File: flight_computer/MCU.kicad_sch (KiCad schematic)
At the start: 43 parts, among them J1 Conn_02x05_Odd_Even, J2 MEM2061-01-188-00-A_REVA, Q1 Q_NPN_BEC, SW1 SW_Push, SW2 SW_Push, U2 STM8S007C8T6TR, Y1 12MHz

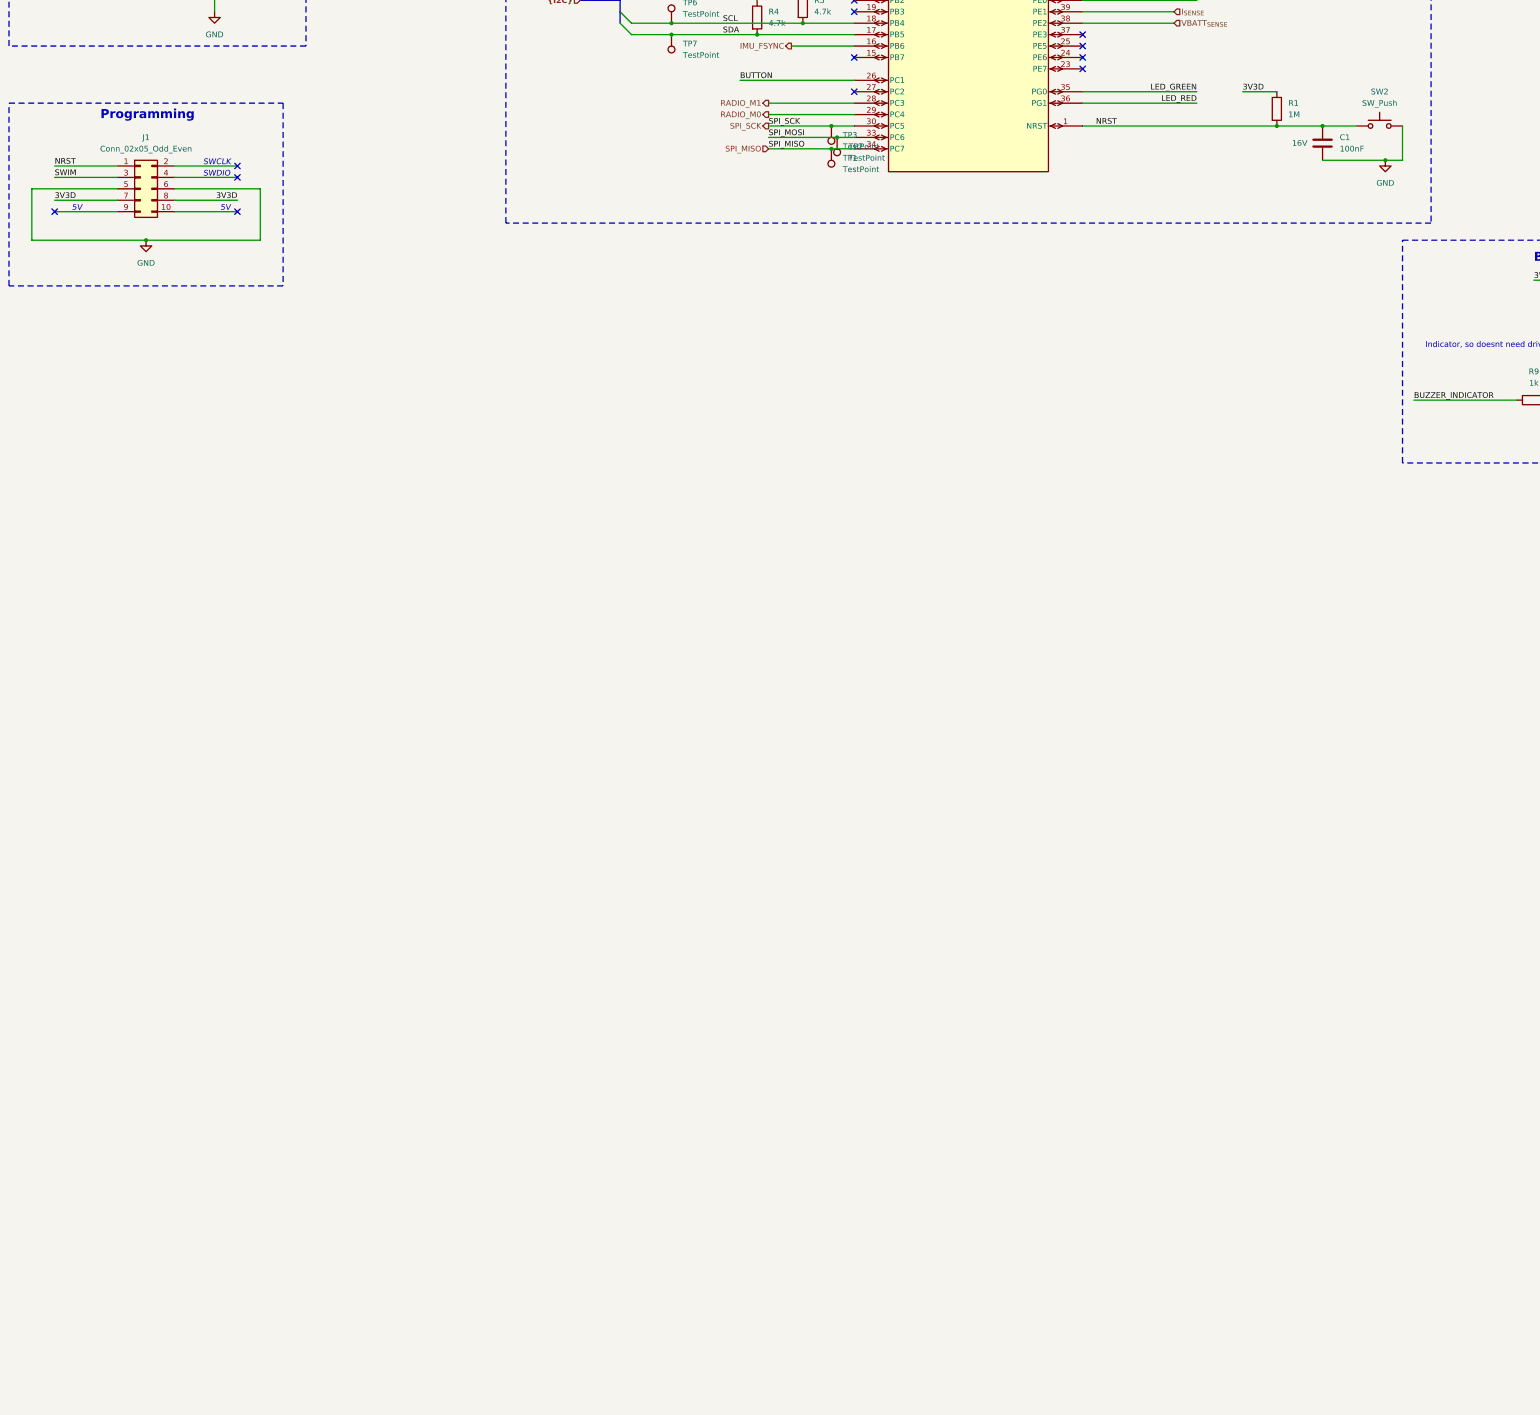
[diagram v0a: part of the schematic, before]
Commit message: start of esp32
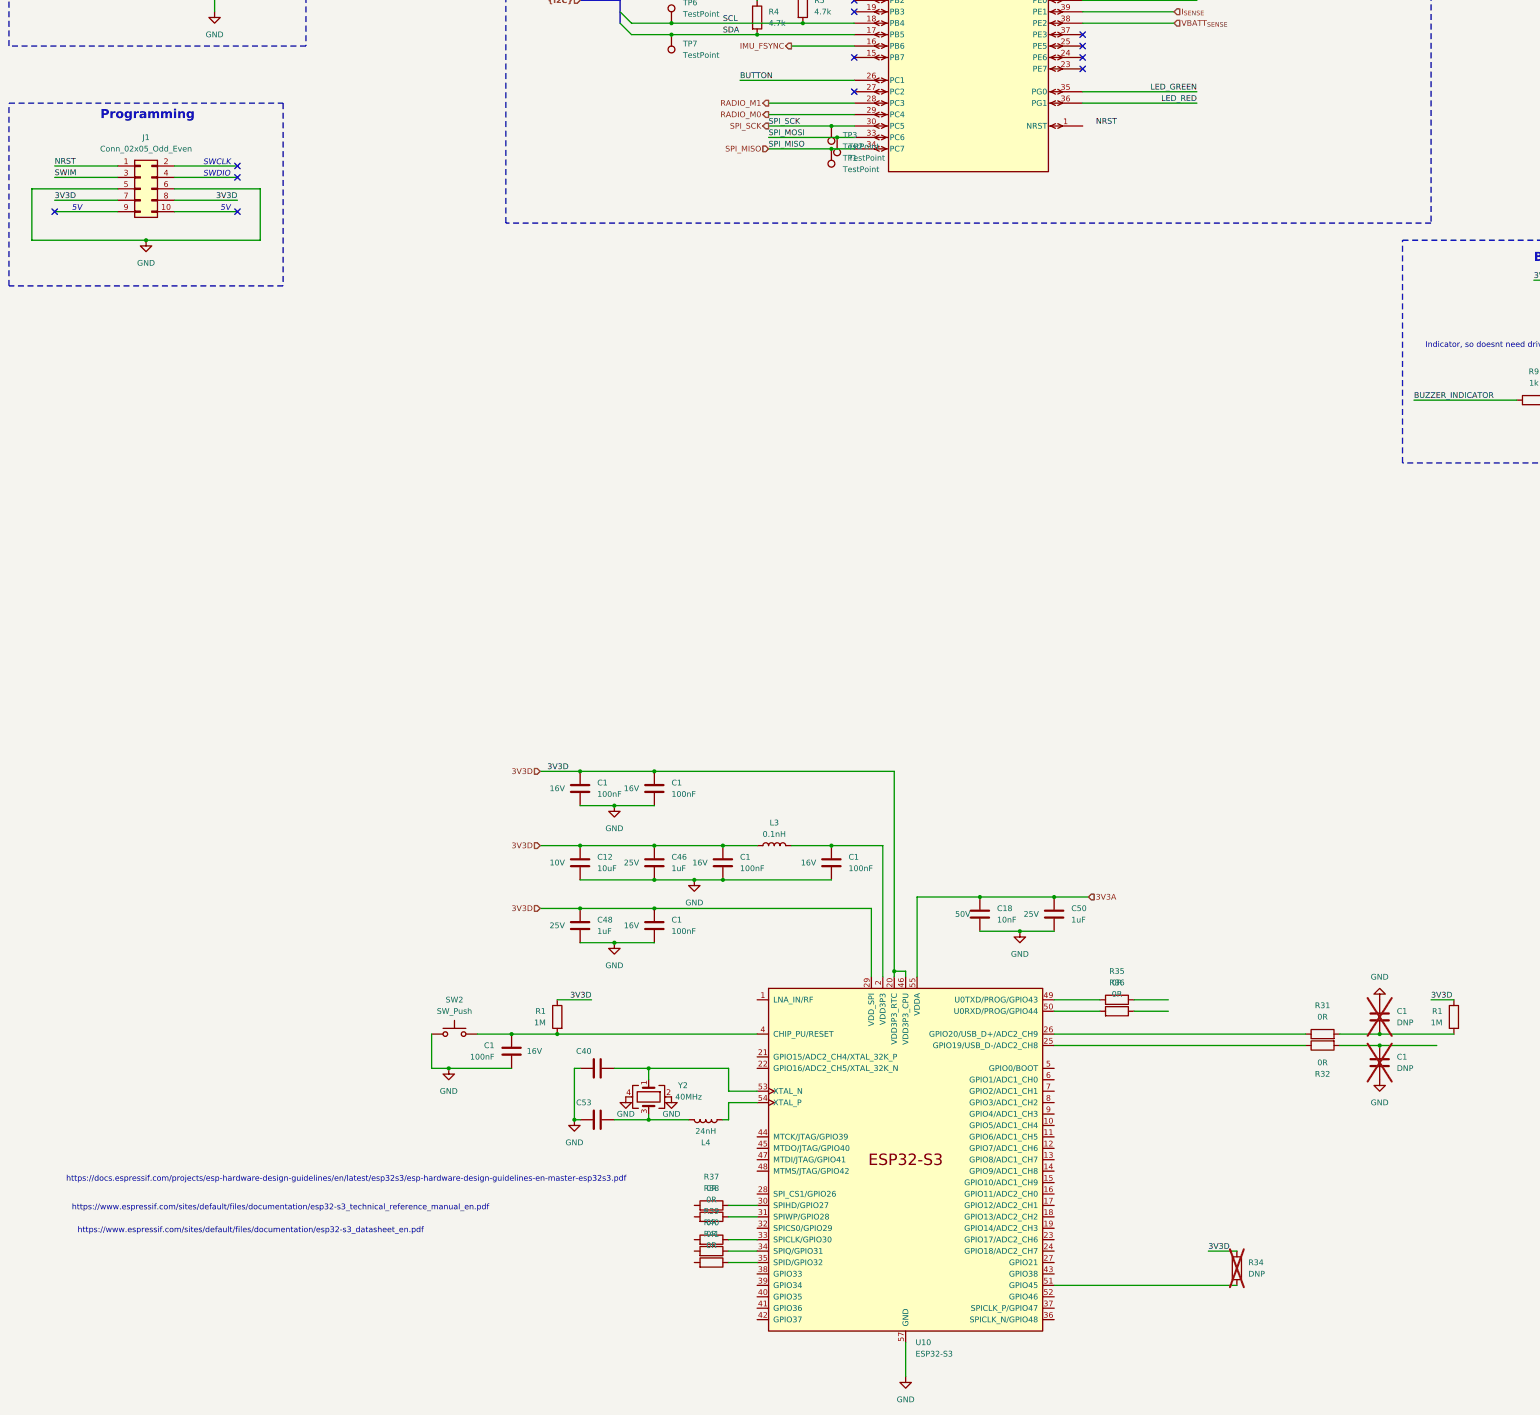
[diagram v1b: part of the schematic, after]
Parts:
- added C1 (x5): 100nF, Capacitor_SMD:C_0402_1005Metric, symbol Device:C
- added C1 (x2): DNP, Capacitor_SMD:C_0402_1005Metric, symbol Device:C
- added C12: 10uF, Capacitor_SMD:C_0402_1005Metric, symbol Device:C
- added C18: 10nF, Capacitor_SMD:C_0402_1005Metric, symbol Device:C
- added C40, C53: ~, Capacitor_SMD:C_0402_1005Metric, symbol Device:C
- added C46, C48, C50: 1uF, Capacitor_SMD:C_0402_1005Metric, symbol Device:C
- added L3: 0.1nH, symbol Device:L
- added L4: 24nH, symbol Device:L
- added R1: 1M, Resistor_SMD:R_0402_1005Metric, symbol Device:R
- added R31, R32, R35, R36, R37, R38, R39, R40, R41: 0R, Resistor_SMD:R_0402_1005Metric, symbol Device:R
- added R34: DNP, Resistor_SMD:R_0402_1005Metric, symbol Device:R
- added U10: ESP32-S3, Package_DFN_QFN:QFN-56-1EP_7x7mm_P0.4mm_EP5.6x5.6mm, symbol Espressif:ESP32-S3
- added Y2: 40MHz, Crystal:Crystal_SMD_3225-4Pin_3.2x2.5mm, symbol Device:Crystal_GND24
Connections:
- net 3V3A: now also C18.1, C50.1, U10.55 (VDDA), U10.56 (VDDA)
- net 3V3D: now also C1.1, C1.1, C1.1, C1.1, C12.1, C46.1, C48.1, L3.1, R1.1, R34.2, U10.20 (VDD3P3_RTC), U10.29 (VDD_SPI), U10.46 (VDD3P3_CPU)
- net GND: now also C1.1, C1.2, C1.2, C1.2, C1.2, C1.2, C1.2, C12.2, C18.2, C40.1, C46.2, C48.2, C50.2, C53.1, U10.57 (GND), Y2.2, Y2.4
- net NRST: no longer C1.1, R1.2, SW2.1, U2.1 (NRST)
- new net: C1.1, R1.2, SW2.1, U10.4 (CHIP_PU/RESET)
- new net: R37.1, U10.30 (SPIHD/GPIO27)
- new net: C53.2, L4.1, Y2.3
- new net: L4.2, U10.54 (XTAL_P)
- new net: C1.2, R1.2, R31.2
- new net: R31.1, U10.26 (GPIO20/USB_D+/ADC2_CH9)
- new net: R32.1, U10.25 (GPIO19/USB_D-/ADC2_CH8)
- new net: C1.1, R32.2
- new net: R38.1, U10.31 (SPIWP/GPIO28)
- new net: R34.1, U10.51 (GPIO45)
- new net: C40.2, U10.53 (XTAL_N), Y2.1
- new net: R39.1, U10.33 (SPICLK/GPIO30)
- new net: R40.1, U10.34 (SPIQ/GPIO31)
- new net: R41.1, U10.35 (SPID/GPIO32)
- new net: R35.2, U10.49 (U0TXD/PROG/GPIO43)
- new net: R36.2, U10.50 (U0RXD/PROG/GPIO44)
- new net VDD3P3: C1.1, L3.2, U10.2 (VDD3P3), U10.3 (VDD3P3)
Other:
- note added: "https://docs.espressif.com/projects/esp-hardware-design-guidelines/en/latest/esp32s3/esp-hardware-design-guidelines-en-master-esp32s3.pdf"
- note added: "https://www.espressif.com/sites/default/files/documentation/esp32-s3_datasheet_en.pdf"
- note added: "https://www.espressif.com/sites/default/files/documentation/esp32-s3_technical_reference_manual_en.pdf"
- moved on the sheet: C1, R1, SW2
